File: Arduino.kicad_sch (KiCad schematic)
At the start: 0 parts

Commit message: new
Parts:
- added A1: Arduino_UNO_R3, Module:Arduino_UNO_R3, symbol MCU_Module:Arduino_UNO_R3
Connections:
- new net AR_A0: A1.9 (A0)
- new net AR_A1: A1.10 (A1)
- new net AR_A2: A1.11 (A2)
- new net AR_A3: A1.12 (A3)
- new net AR_A4: A1.13 (SDA/A4)
- new net AR_A5: A1.14 (SCL/A5)
- new net AR_D2: A1.17 (D2)
- new net AR_D3: A1.18 (D3)
- new net AR_D4: A1.19 (D4)
- new net AR_D5: A1.20 (D5)
- new net AR_D6: A1.21 (D6)
- new net AR_D7: A1.22 (D7)
- new net AR_D8: A1.23 (D8)
- new net AR_D9: A1.24 (D9)
- new net AR_MISO: A1.27 (D12)
- new net AR_MOSI: A1.26 (D11)
- new net AR_RX: A1.16 (D1/TX)
- new net AR_SCK: A1.28 (D13)
- new net AR_SCL: A1.32 (SCL/A5)
- new net AR_SDA: A1.31 (SDA/A4)
- new net AR_SS: A1.25 (D10)
- new net AR_TX: A1.15 (D0/RX)
- new net GND: A1.29 (GND), A1.6 (GND), A1.7 (GND)
- new net VIN: A1.8 (VIN)
- no-connect marks 0 -> 5

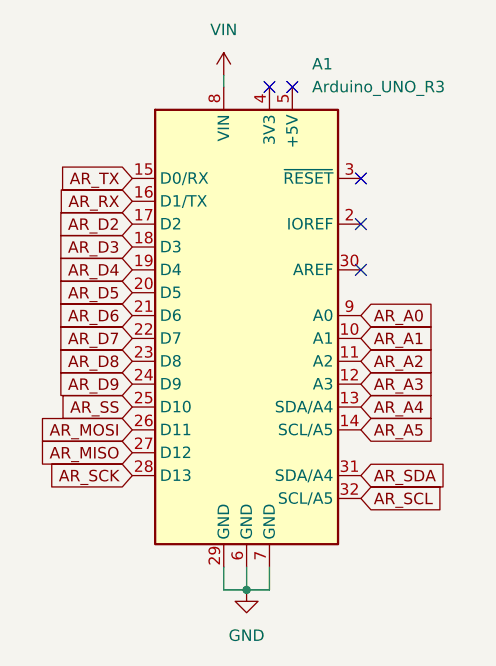
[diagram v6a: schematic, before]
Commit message: new
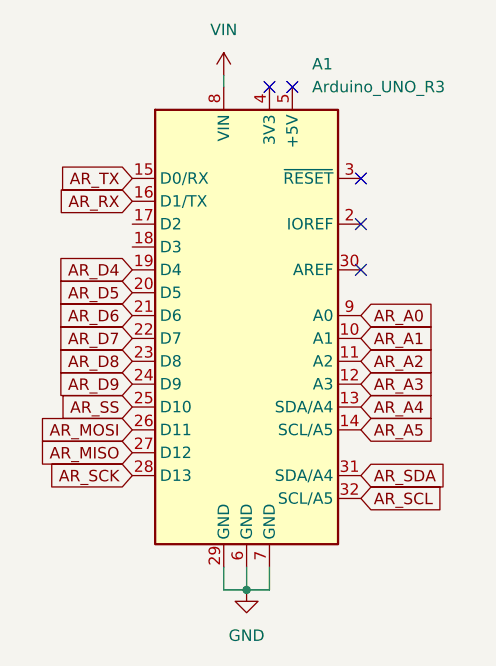
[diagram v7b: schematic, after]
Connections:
- net AR_D2: no longer names the net of A1.17 (D2)
- net AR_D3: no longer names the net of A1.18 (D3)
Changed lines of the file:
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@@
-		)
-	)
-	(global_label "AR_D3"
-		(shape input)
-		(at 132.08 82.55 180)
-		(fields_autoplaced yes)
-		(effects
-			(font
-				(size 1.27 1.27)
-			)
-			(justify right)
-		)
-		(property "Intersheetrefs" "${INTERSHEET_REFS}"
-			(at 123.2891 82.55 0)
-			(effects
-				(font
-					(size 1.27 1.27)
-				)
-				(justify right)
-				(hide yes)
-			)
 		)
 	)
@@
 			(effects
 				(font
-					(size 1.27 1.27)
-				)
-				(justify right)
-				(hide yes)
-			)
-		)
-	)
-	(global_label "AR_D2"
-		(shape input)
-		(at 132.08 80.01 180)
-		(fields_autoplaced yes)
-		(effects
-			(font
-				(size 1.27 1.27)
-			)
-			(justify right)
-		)
-		(property "Intersheetrefs" "${INTERSHEET_REFS}"
-			(at 123.2891 80.01 0)
-			(effects
-				(font
